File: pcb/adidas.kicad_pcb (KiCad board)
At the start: 2 copper layers, 152.7 x 107.2 mm, 32 parts, among them J1 ISP Header, J2 Shitty Add-on, J4 Battery, U1 MPU-6050, U2 ATTINY841-SSU

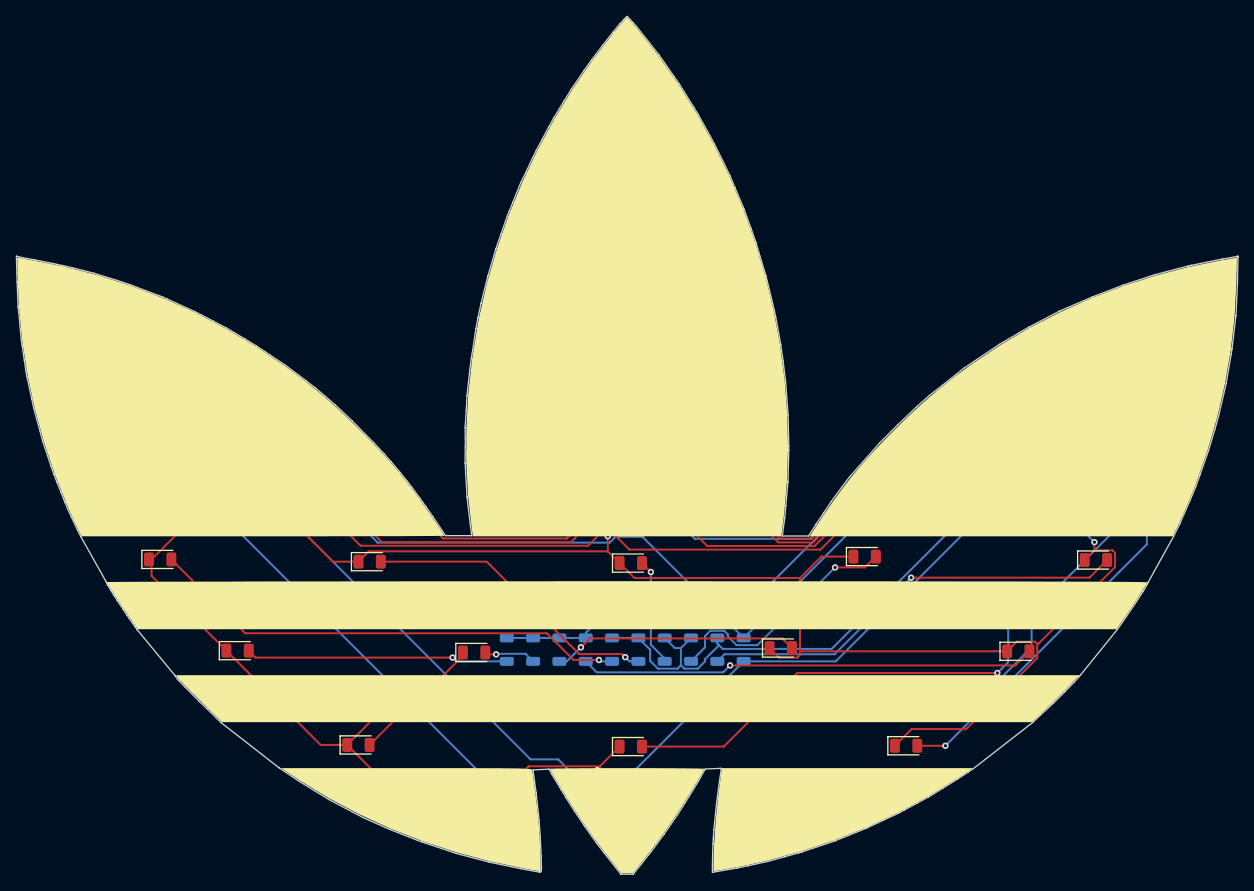
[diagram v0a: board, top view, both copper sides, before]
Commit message: run ERC checks
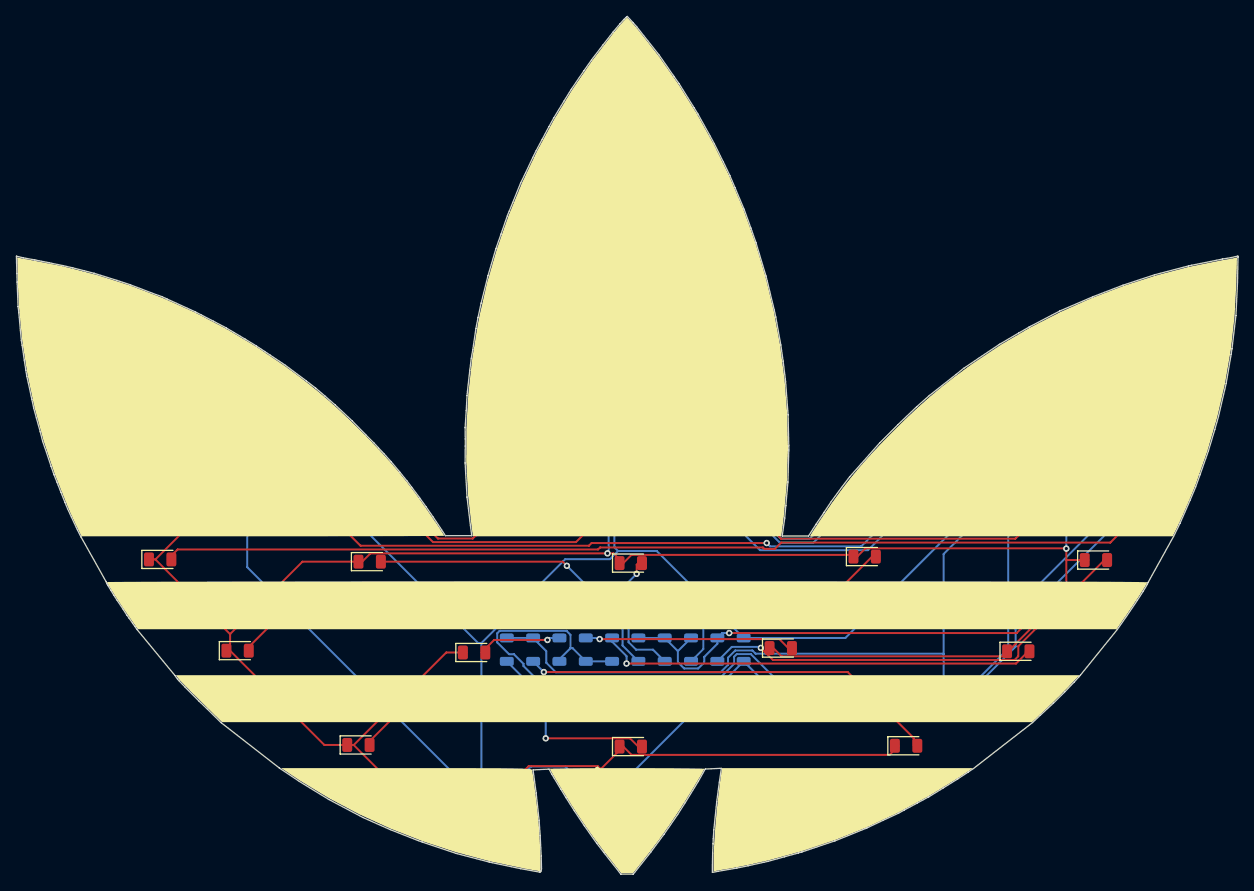
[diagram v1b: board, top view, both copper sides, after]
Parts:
- D1, D10, D11, D12, D2, D3, D4, D5, D6, D7, D8, D9: value CTL1206FWH1T -> AP3216SYCK
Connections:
- R2 pad 1: /2(LED Bottom Row) -> Net-(D4-Pad2)
- R2 pad 2: Net-(D2-Pad2) -> /3(LED Mid Row)
- R3 pad 1: /2(LED Bottom Row) -> /5(LED Top Row)
- R3 pad 2: Net-(D3-Pad2) -> Net-(D8-Pad2)
- R4 pad 1: /3(LED Mid Row) -> /2(LED Bottom Row)
- R4 pad 2: Net-(D4-Pad2) -> Net-(D2-Pad2)
- R5 pad 1: /3(LED Mid Row) -> /2(LED Bottom Row)
- R5 pad 2: Net-(D5-Pad2) -> Net-(D3-Pad2)
- R6 pad 1: /3(LED Mid Row) -> Net-(D5-Pad2)
- R6 pad 2: Net-(D6-Pad2) -> /3(LED Mid Row)
- R7 pad 1: /3(LED Mid Row) -> Net-(D6-Pad2)
- R7 pad 2: Net-(D7-Pad2) -> /3(LED Mid Row)
- R8 pad 1: /5(LED Top Row) -> Net-(D7-Pad2)
- R8 pad 2: Net-(D8-Pad2) -> /3(LED Mid Row)
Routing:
- net Net-(D4-Pad2): track 32.8 -> 100.2 mm
- net Net-(D8-Pad2): track 60.4 -> 124.8 mm
- net (no net): track 0.00 -> 59.2 mm
- net /2(LED Bottom Row): track 51.9 -> 101.6 mm
- net /3(LED Mid Row): track 92.7 -> 127.5 mm, vias 2 -> 0
- net Net-(D2-Pad2): track 56.2 -> 23.6 mm
- net VCC: track 179.4 -> 149.7 mm
- net /7(SDA): track 161.3 -> 189.3 mm, vias 1 -> 0
- net /4(RST): track 147.6 -> 169.9 mm
- net GND: track 347.2 -> 367.1 mm
- net Net-(D3-Pad2): track 42.6 -> 52.5 mm
- net Net-(J1-Pin_1): track 116.4 -> 121.6 mm
- net Net-(D6-Pad2): track 30.7 -> 25.8 mm
- net Net-(D5-Pad2): track 6.50 -> 10.5 mm
- net Net-(D7-Pad2): track 57.1 -> 54.7 mm
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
